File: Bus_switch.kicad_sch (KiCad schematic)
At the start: 15 parts, among them J3 Conn_01x04_Pin, U3 SN74CB3Q3245PWR

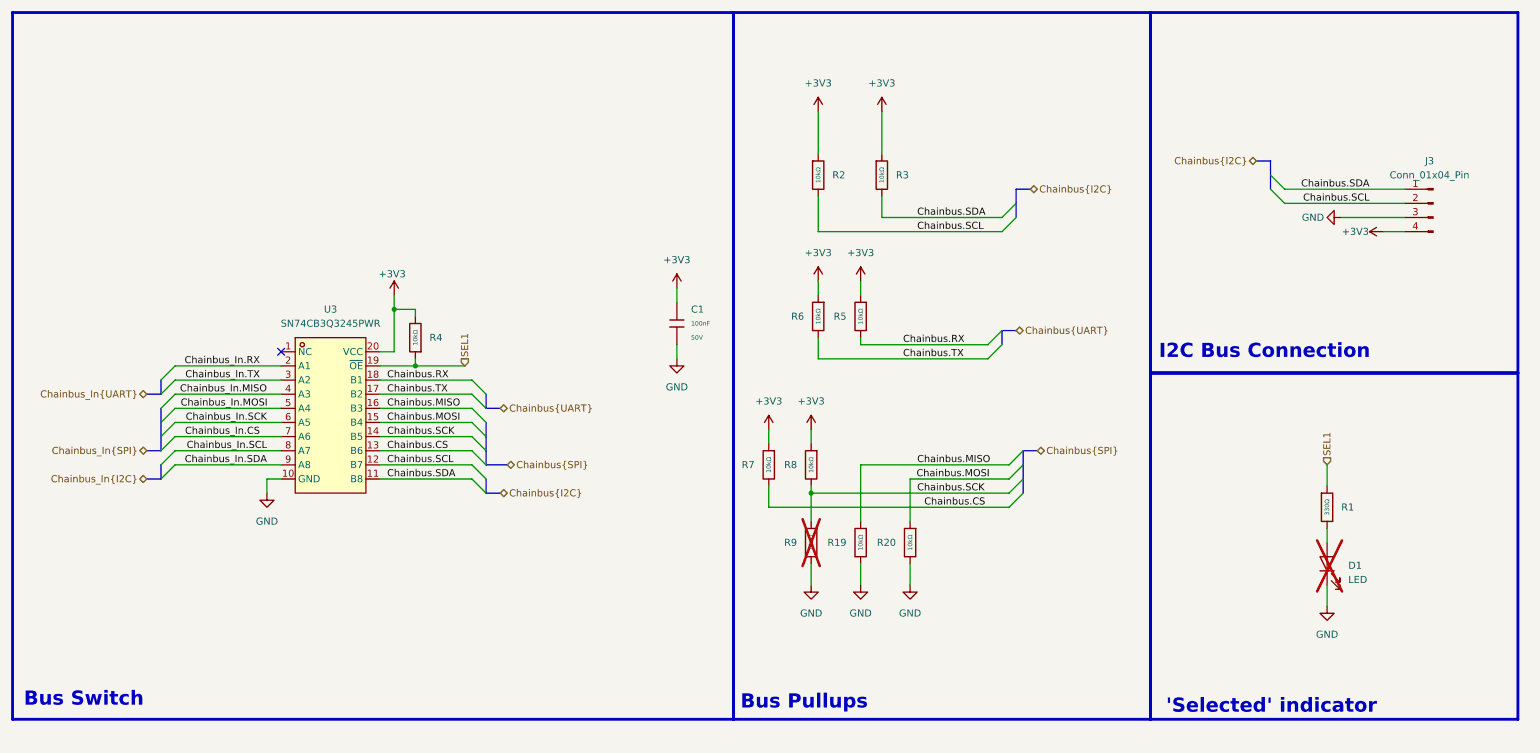
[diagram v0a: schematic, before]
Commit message: polished the schemtic
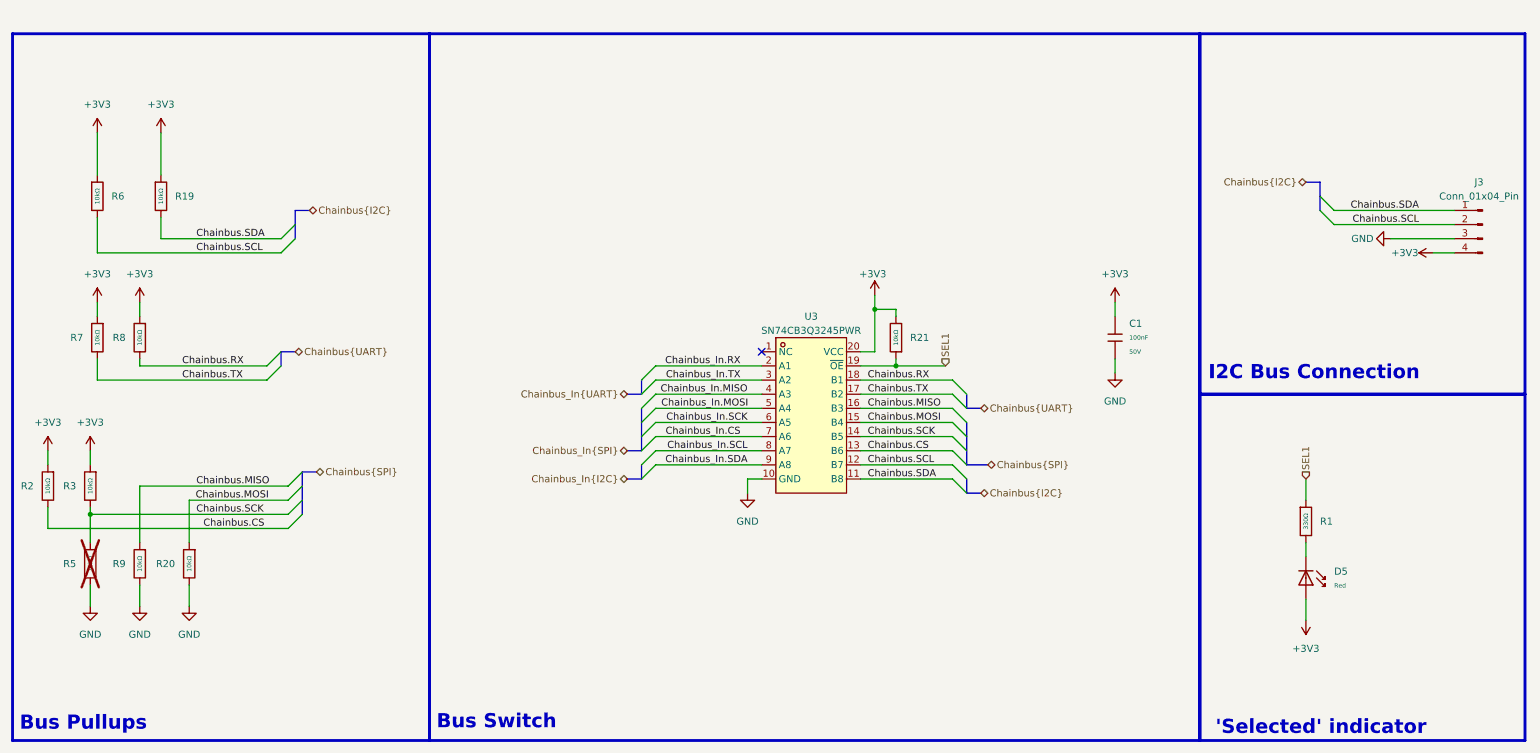
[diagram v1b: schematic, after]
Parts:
- removed D1: LED, LED_SMD:LED_0603_1608Metric, symbol Device:LED
- removed R4: 10kΩ, PCM_JLCPCB:R_0402, symbol PCM_JLCPCB-Resistors:0402,10kΩ
- added D5: Red, PCM_JLCPCB:D_0603, symbol PCM_JLCPCB-Diodes:LED,0603,Red
- added R21: 10kΩ, PCM_JLCPCB:R_0402, symbol PCM_JLCPCB-Resistors:0402,10kΩ
- R5: now not fitted; now left out of the parts list
- R9: now fitted; now in the parts list
- U3: TME (none) -> SN74CB3Q3245PWR
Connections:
- net +3V3: now also R19.1, D5.2, R21.2; no longer R5.1
- net Chainbus.CS: now also R2.2; no longer R7.2
- net Chainbus.MISO: now also R9.1; no longer R19.1
- net Chainbus.RX: now also R8.2; no longer R5.2
- net Chainbus.SCK: now also R3.2, R5.1; no longer R8.2, R9.1
- net Chainbus.SCL: now also R6.2; no longer R2.2
- net Chainbus.SDA: now also R19.2; no longer R3.2
- net Chainbus.TX: now also R7.2; no longer R6.2
- net GND: now also R5.2; no longer R19.2
- net SEL1: now also R21.1
- net at R1.2: now also D5.1
